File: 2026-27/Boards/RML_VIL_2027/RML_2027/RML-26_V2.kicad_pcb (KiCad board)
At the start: 2 copper layers, 90.1 x 30 mm, 27 parts, among them J1 043045-0412, Q2 AO3401A, Q3 UJ3N065080K3S, Q4 AO3401A, U1 H11L1M, U2 NE555D

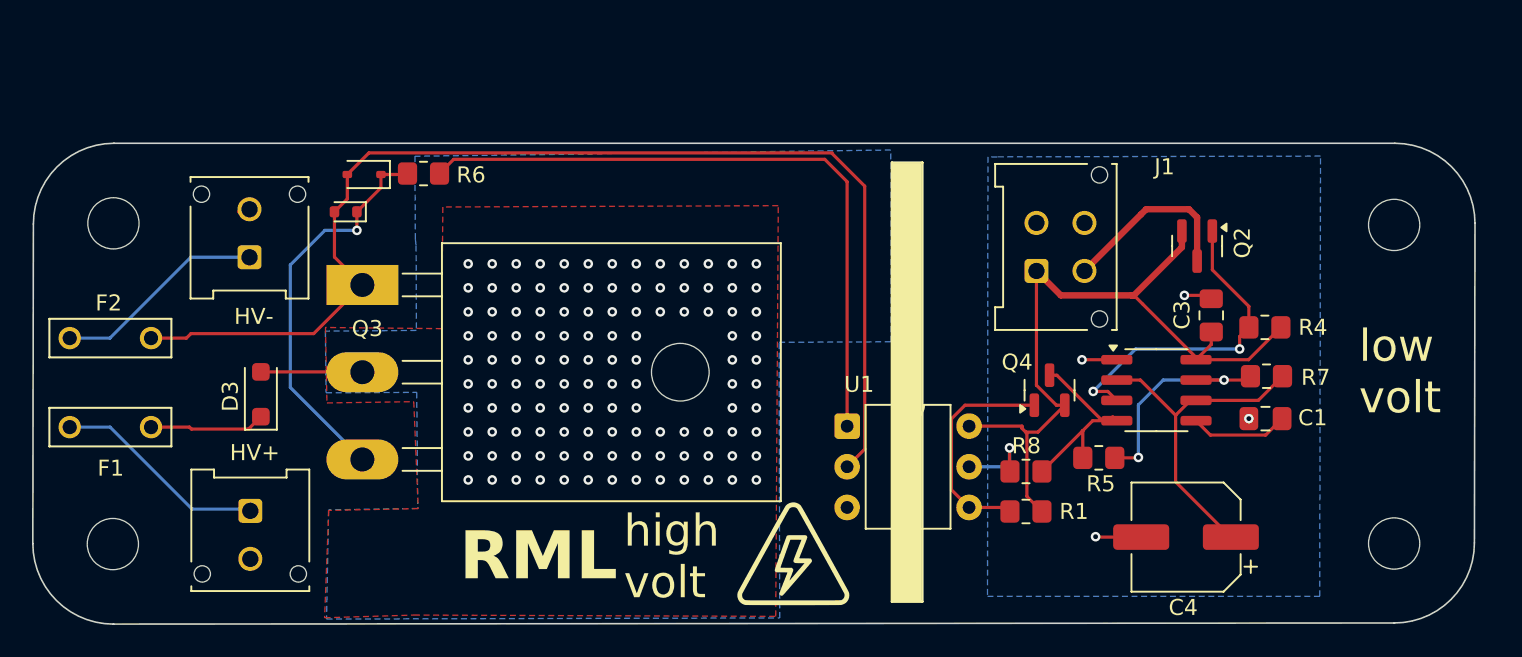
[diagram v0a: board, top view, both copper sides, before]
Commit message: pcb trace
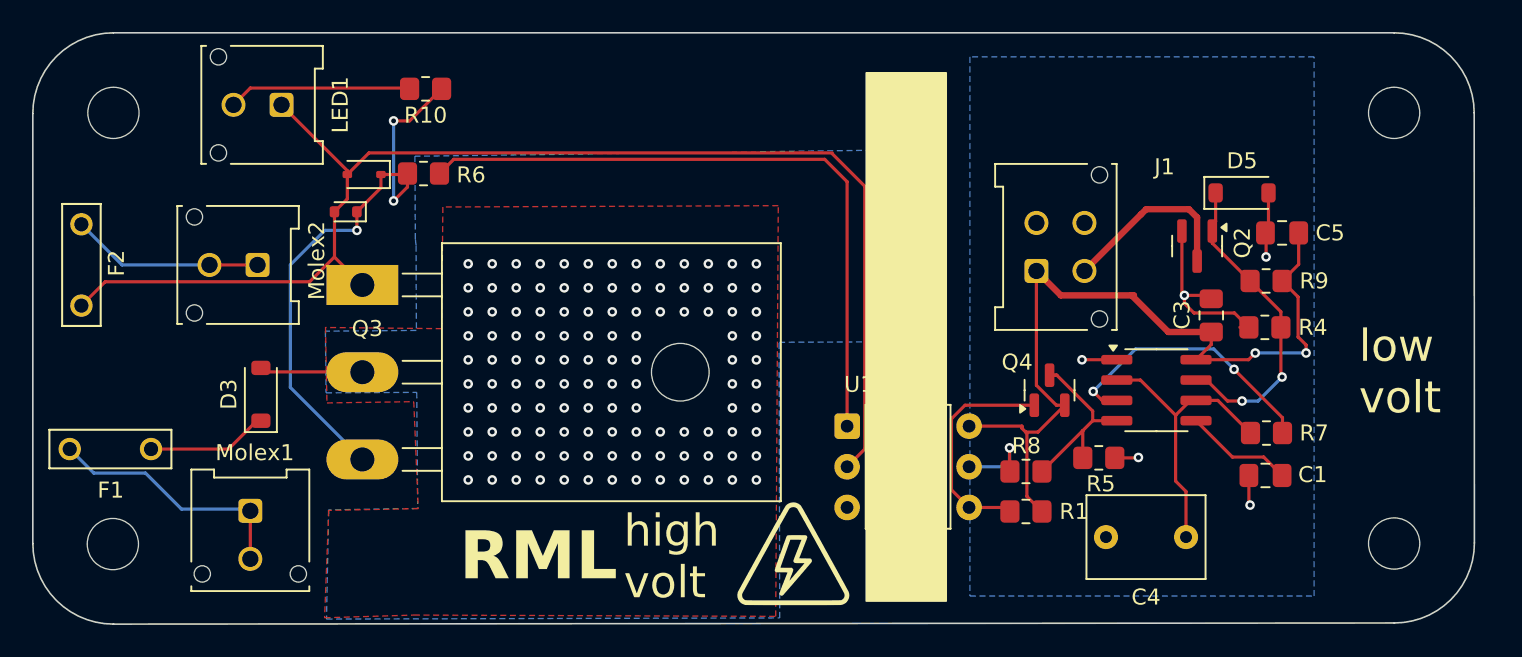
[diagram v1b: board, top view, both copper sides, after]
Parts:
- added C5: 100nF, Capacitor_SMD:C_0805_2012Metric_Pad1.18x1.45mm_HandSolder, F.Cu at (182.0, 81.1)
- added D5: BZT52C8V2, Diode_SMD:D_SOD-123, F.Cu at (179.5, 78.6)
- added LED1: 043045-0212, Connector_Molex:Molex_Micro-Fit_3.0_43045-0212_2x01_P3.00mm_Vertical, F.Cu at (119.5, 73.1)
- added R10: 1k, Resistor_SMD:R_0805_2012Metric_Pad1.20x1.40mm_HandSolder, F.Cu at (128.5, 72.1)
- added R9: 10k, Resistor_SMD:R_0805_2012Metric_Pad1.20x1.40mm_HandSolder, F.Cu at (181.0, 84.1)
- C4: value 100uF -> 1uF film; footprint Capacitor_SMD:CP_Elec_6.3x5.4 -> Capacitor_THT:C_Rect_L7.2mm_W5.0mm_P5.00mm
- D1: value 1N4148WT -> 1N4148WT-7
- D3: value BZT52C51 -> BZT52C51-7-F; footprint Diode_SMD:D_SOD-123F -> Diode_SMD:D_SOD-123
- Q2: value AO3401A -> AO3400A
- R4: value 1k -> 100k
- R7: value 3k -> 750k
- U1: value H11L1M -> H11L1
- U2: value NE555D -> LMC555CMX/NOPB
- moved H1 7.00 mm to (189.0, 73.6)
- moved H3 6.90 mm to (109.0, 73.6)
- moved F2 4.92 mm to (107.0, 83.1), turned to 90 degrees
- moved C1 3.55 mm to (181.0, 96.2)
- moved R7 3.55 mm to (181.0, 93.6), turned to 0 degrees
- moved F1 1.37 mm to (108.8, 94.6)
- moved Molex2 0.69 mm to (118.0, 83.1), turned to -90 degrees
- renumbered HV+ to Molex1, HV- to Molex2
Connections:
- net Light+ renamed LED_RETURN
- Molex1 pad 2: unconnected-(Molex1-Pin_2-Pad2) -> /HV+
- Molex2 pad 2: unconnected-(Molex2-Pin_2-Pad2) -> Net-(Molex2-Pin_1)
- Q2 pad 1: Net-(Q2-G) -> Net-(D5-K)
- Q2 pad 2: GLV+ -> GND
- R4 pad 1: Net-(Q2-G) -> GND
- R4 pad 2: GLV+ -> Net-(D5-K)
- R7 pad 2: Net-(U2-DIS) -> Net-(U2-Q)
- U2 pad 3: Net-(Q2-G) -> Net-(U2-Q)
- U2 pad 7: Net-(U2-DIS) -> Net-(D5-K)
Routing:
- net Net-(Q2-G): track 20.5 -> 0.00 mm, vias 2 -> 0
- net Net-(D5-K): track 0.00 -> 19.1 mm, vias 0 -> 2
- net Net-(U2-Q): track 0.00 -> 17.4 mm, vias 0 -> 2
- net GND: track 11.8 -> 25.4 mm
- net Net-(U2-DIS): track 14.3 -> 1.49 mm, vias 2 -> 1
- net Net-(LED1-Pin_2): track 0.00 -> 11.5 mm
- net Net-(D1-K): track 24.9 -> 35.8 mm, vias 1 -> 3
- net /HV-: track 74.2 -> 83.8 mm
- net GLV+: track 47.7 -> 52.4 mm, vias 0 -> 2
- net Net-(U2-THR): track 21.3 -> 18.4 mm
- net /HV+: track 13.5 -> 15.9 mm
- net Net-(Molex2-Pin_1): track 13.3 -> 12.1 mm
- net Net-(U2-CV): track 6.17 -> 6.79 mm
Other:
- board size 90.1 x 30 mm -> 90.1 x 36.9 mm
